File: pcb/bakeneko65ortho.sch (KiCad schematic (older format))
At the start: 164 parts, among them J1 1x4P 1mm, J2 AVR-ISP-6, SW1 SW_Push, U1 ATmega32U4-AU, U2 SRV05-4, Y1 16MHz

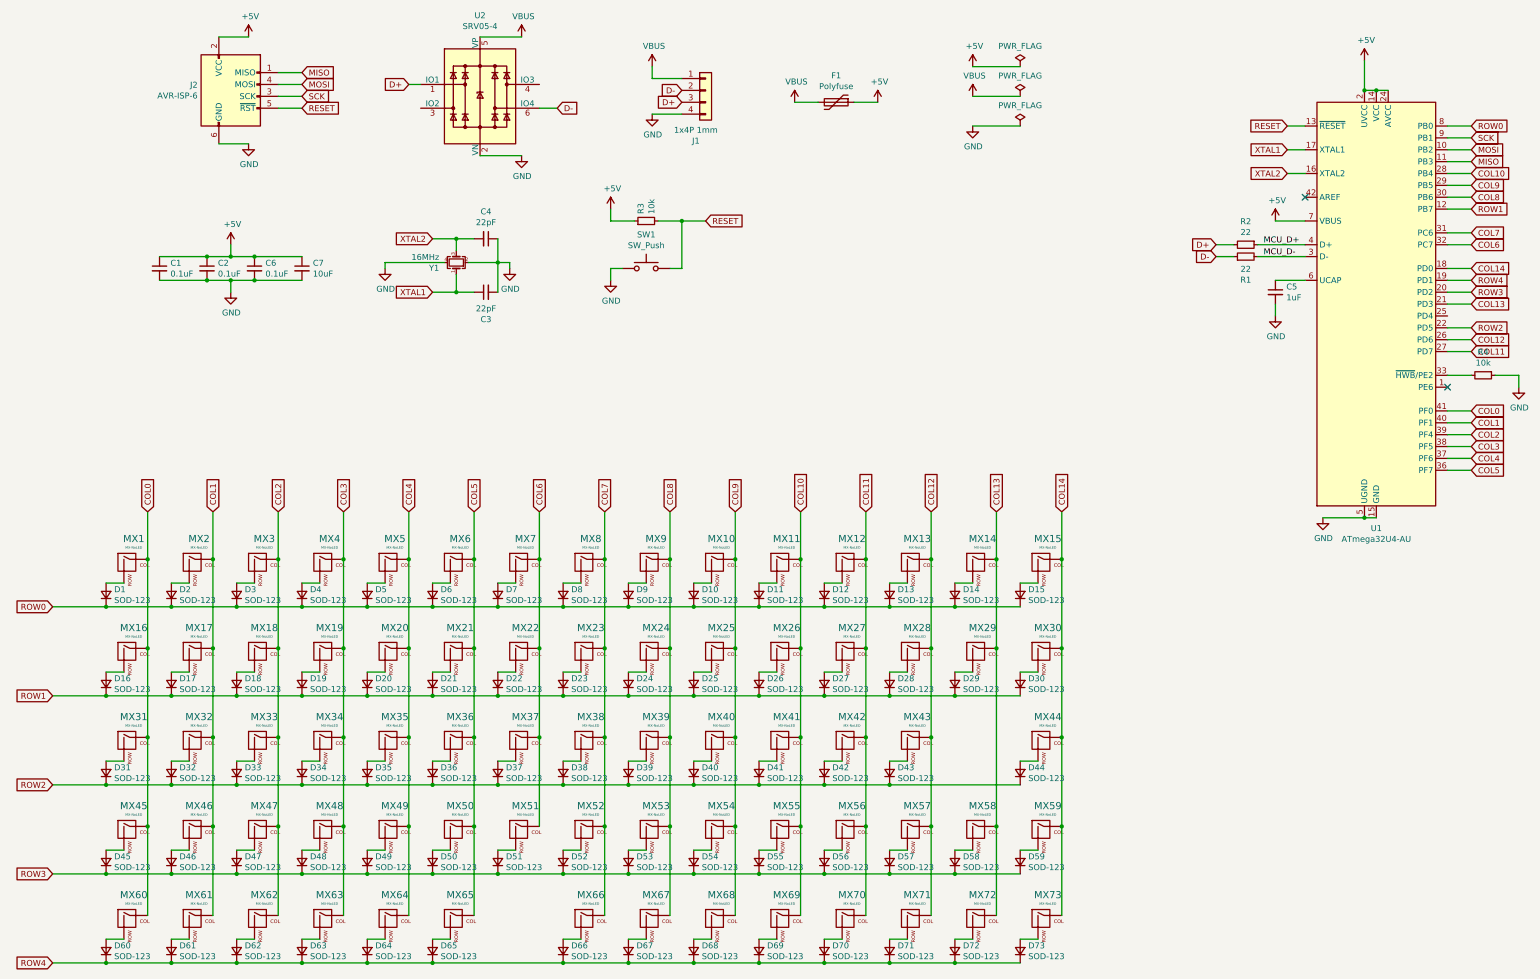
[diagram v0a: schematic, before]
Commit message: add graphics
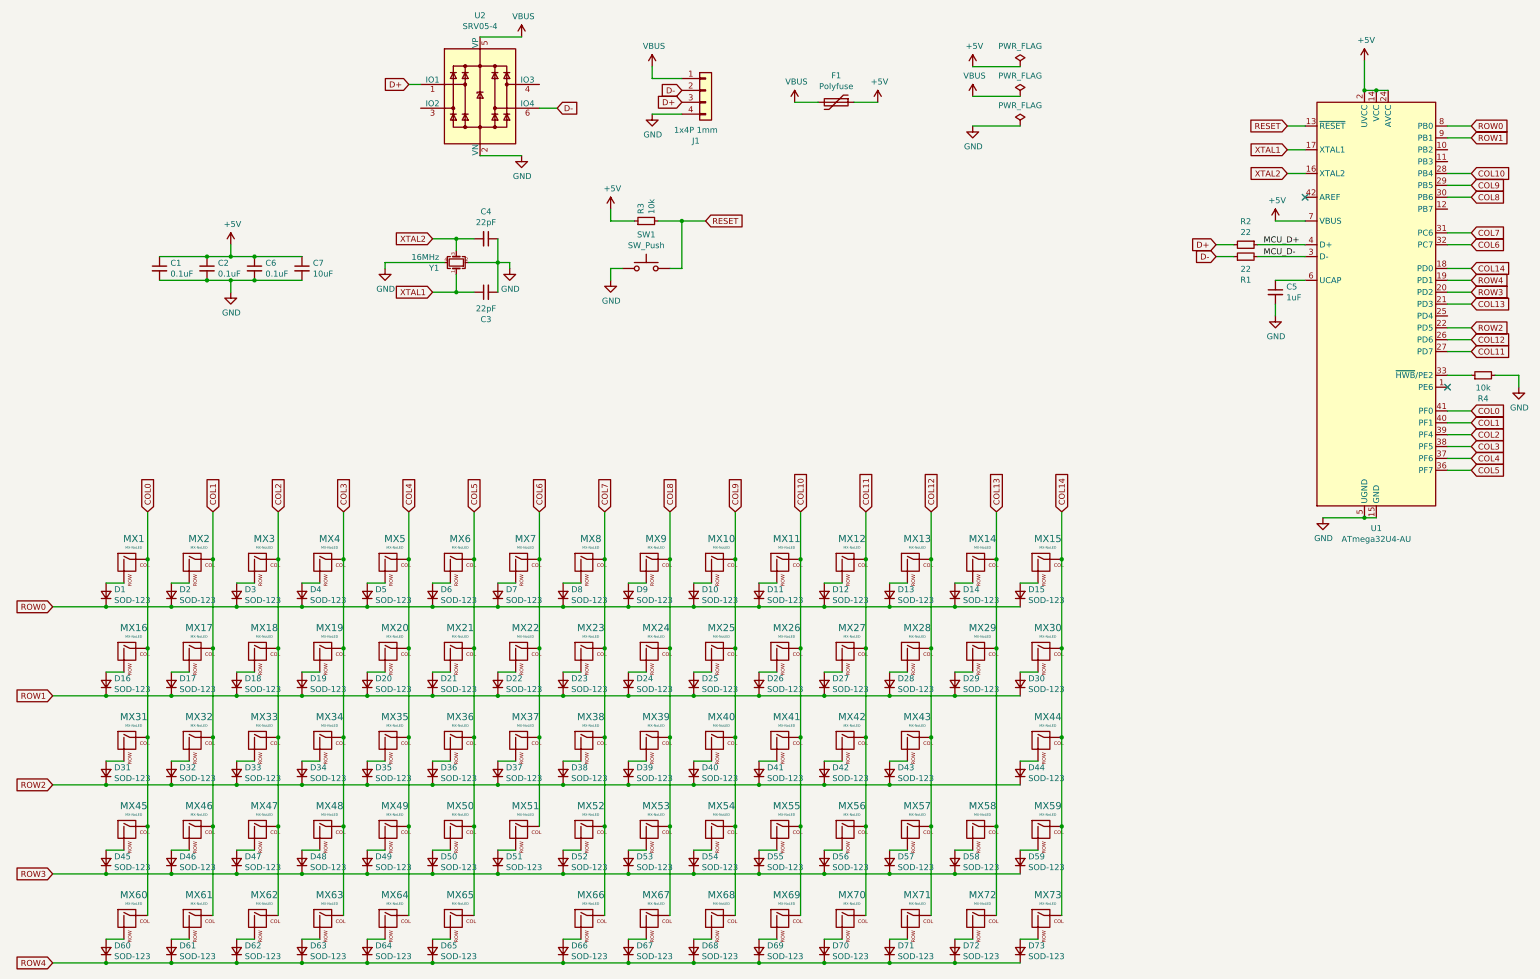
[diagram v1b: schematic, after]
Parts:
- removed J2: AVR-ISP-6, bakeneko:ISP, symbol Connector:AVR-ISP-6
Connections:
- net SCK is gone; now on net ROW1: U1.9 (PB1)
- net GND: now also R4.2; no longer R4.1
- net ROW1: no longer U1.12 (PB7)
- net at U1.33 (~HWB~/PE2): now also R4.1; no longer R4.2
- net MISO: no longer names the net of U1.11 (PB3)
- net MOSI: no longer names the net of U1.10 (PB2)
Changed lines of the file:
@@
 F 3 "~" H 13450 5650 50  0001 C CNN
 	1    13450 5650
-	0    1    1    0
+	0    -1   -1   0
 $EndComp
 $Comp
@@
 Text GLabel 13350 5050 2    50   Input ~ 0
 COL13
-Text GLabel 13350 4250 2    50   Input ~ 0
+Text GLabel 13350 3650 2    50   Input ~ 0
 ROW1
 Text GLabel 13350 3550 2    50   Input ~ 0
@@
 Wire Wire Line
 	13150 4950 13350 4950
-$Comp
-L Connector:AVR-ISP-6 J2
-U 1 1 629205EC
-P 2900 3300
-F 0 "J2" H 2621 3396 50  0000 R CNN
-F 1 "AVR-ISP-6" H 2621 3305 50  0000 R CNN
-F 2 "bakeneko:ISP" V 2650 3350 50  0001 C CNN
-F 3 " ~" H 1625 2750 50  0001 C CNN
-	1    2900 3300
-	1    0    0    -1
-$EndComp
-$Comp
-L power:+5V #PWR0111
-U 1 1 62922AAE
-P 3050 2800
-F 0 "#PWR0111" H 3050 2650 50  0001 C CNN
-F 1 "+5V" H 3065 2973 50  0000 C CNN
-F 2 "" H 3050 2800 50  0001 C CNN
-F 3 "" H 3050 2800 50  0001 C CNN
-	1    3050 2800
-	1    0    0    -1
-$EndComp
-Wire Wire Line
-	2800 2800 3050 2800
-$Comp
-L power:GND #PWR0112
-U 1 1 6295962C
-P 3050 3700
-F 0 "#PWR0112" H 3050 3450 50  0001 C CNN
-F 1 "GND" H 3055 3527 50  0000 C CNN
-F 2 "" H 3050 3700 50  0001 C CNN
-F 3 "" H 3050 3700 50  0001 C CNN
-	1    3050 3700
-	1    0    0    -1
-$EndComp
-Wire Wire Line
-	2800 3700 3050 3700
-Text GLabel 3500 3100 2    50   Input ~ 0
-MISO
-Text GLabel 3500 3200 2    50   Input ~ 0
-MOSI
-Text GLabel 3500 3300 2    50   Input ~ 0
-SCK
-Text GLabel 3500 3400 2    50   Input ~ 0
-RESET
-Wire Wire Line
-	3300 3100 3500 3100
-Wire Wire Line
-	3300 3200 3500 3200
-Wire Wire Line
-	3300 3300 3500 3300
-Wire Wire Line
-	3300 3400 3500 3400
 $Comp
 L power:PWR_FLAG #FLG0101
@@
 	11700 4350 11950 4350
 NoConn ~ 11950 4150
-Text GLabel 13350 3650 2    50   Input ~ 0
-SCK
 Wire Wire Line
 	13350 3650 13150 3650
-Text GLabel 13350 3750 2    50   Input ~ 0
-MOSI
-Wire Wire Line
-	13350 3750 13150 3750
-Text GLabel 13350 3850 2    50   Input ~ 0
-MISO
-Wire Wire Line
-	13350 3850 13150 3850
-Wire Wire Line
-	13350 4250 13150 4250
 Wire Wire Line
 	13750 5750 13750 5650
